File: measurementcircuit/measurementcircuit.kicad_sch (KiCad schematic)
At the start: 166 parts, among them J1 Conn_01x02, J10 Conn_01x02, J11 Conn_01x02, J12 Conn_01x02, J13 2604-3102, J14 DILB28P-223TLF, J15 Conn_01x02, J16 Conn_01x02, J17 Conn_01x02, J18 2604-3102, J19 2604-3102, J2 Conn_01x02, J20 2604-3102, J21 Conn_01x02, J22 Conn_01x02, J23 Conn_01x02, J24 Conn_01x02, J25 Conn_01x02, J26 Conn_01x02, J27 Conn_01x02, J28 Conn_01x02, J29 Conn_01x02, J3 2604-3102, J30 Conn_01x02, J31 Conn_01x02, J32 Conn_01x02, J33 Conn_01x02, J34 Conn_01x02, J35 Conn_01x02, J36 Conn_01x02, J37 Conn_01x02, J38 Conn_01x02, J39 Conn_01x02, J4 2604-3102, J40 Conn_01x02, J41 Conn_01x02, J42 Conn_01x02, J43 DILB28P-223TLF, J44 2601-1102, J45 2601-1108, J46 2601-1108, J47 Conn_01x02, J48 Conn_01x02, J49 Conn_01x02, J5 2604-3102, J50 2604-3102, J51 Conn_01x02, J52 Conn_01x02, J53 Conn_01x02, J54 Conn_01x02, J55 2604-3102, J56 Conn_01x02, J57 Conn_01x02, J58 Conn_01x02, J59 Conn_01x02, J6 2604-3102, J60 2601-1108, J61 2604-3102, J62 Conn_01x02, J63 Conn_01x02, J64 Conn_01x02, J65 Conn_01x02, J66 2604-3102, J67 Conn_01x02, J68 Conn_01x02, J69 Conn_01x02, J7 2604-3102, J70 Conn_01x02, J71 2604-3102, J72 Conn_01x02, J73 Conn_01x02, J74 Conn_01x02, J75 Conn_01x02, J76 2604-3102, J77 Conn_01x02, J78 Conn_01x02, J79 Conn_01x02, J8 Conn_01x02, J80 Conn_01x02, J81 2604-3102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

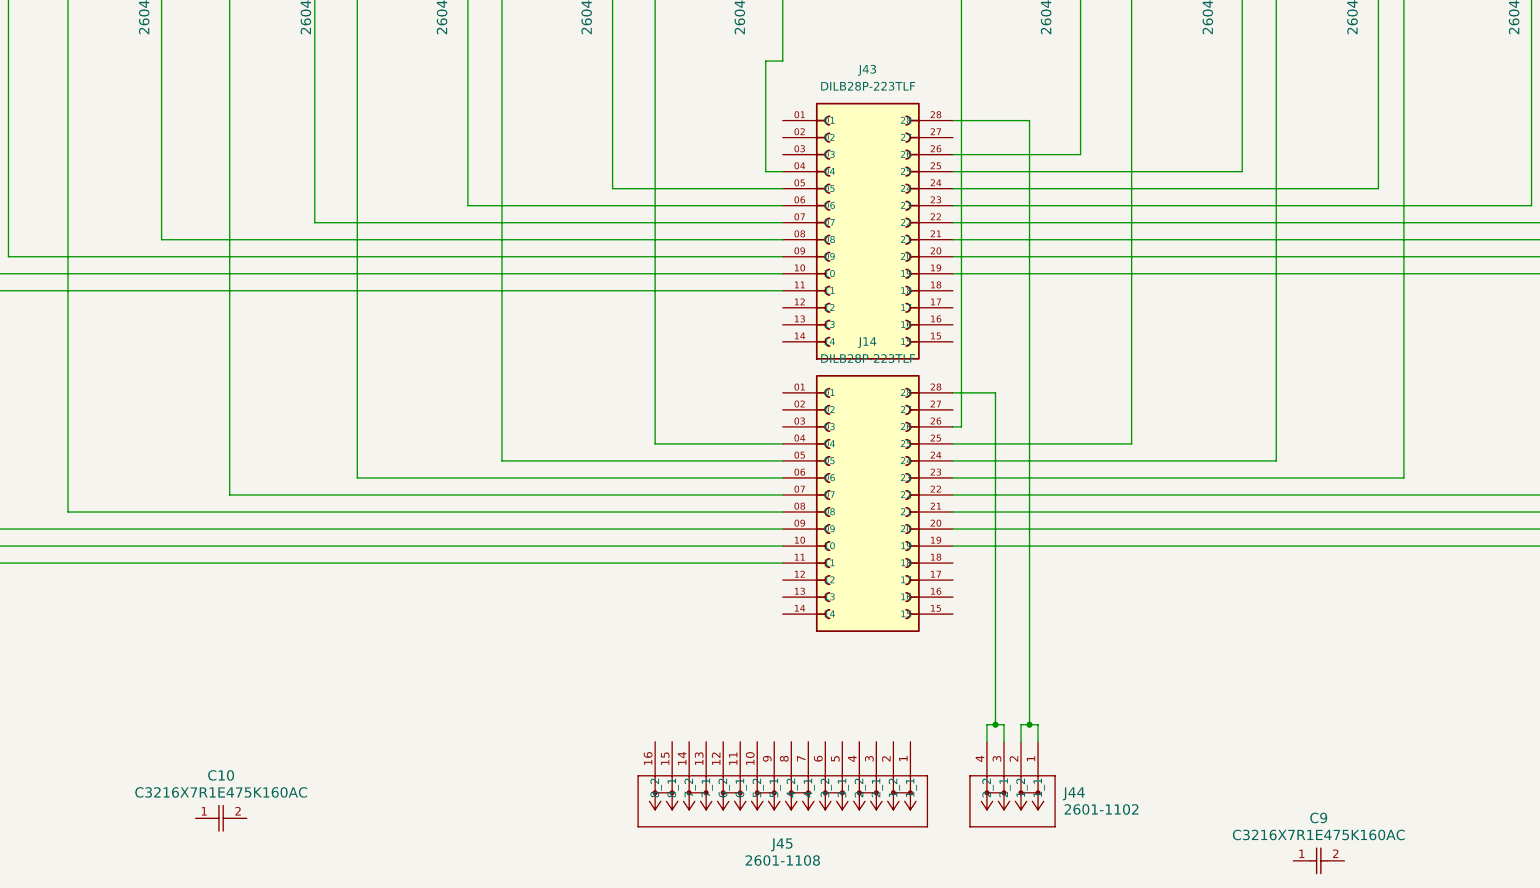
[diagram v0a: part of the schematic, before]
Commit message: Schematic Complete
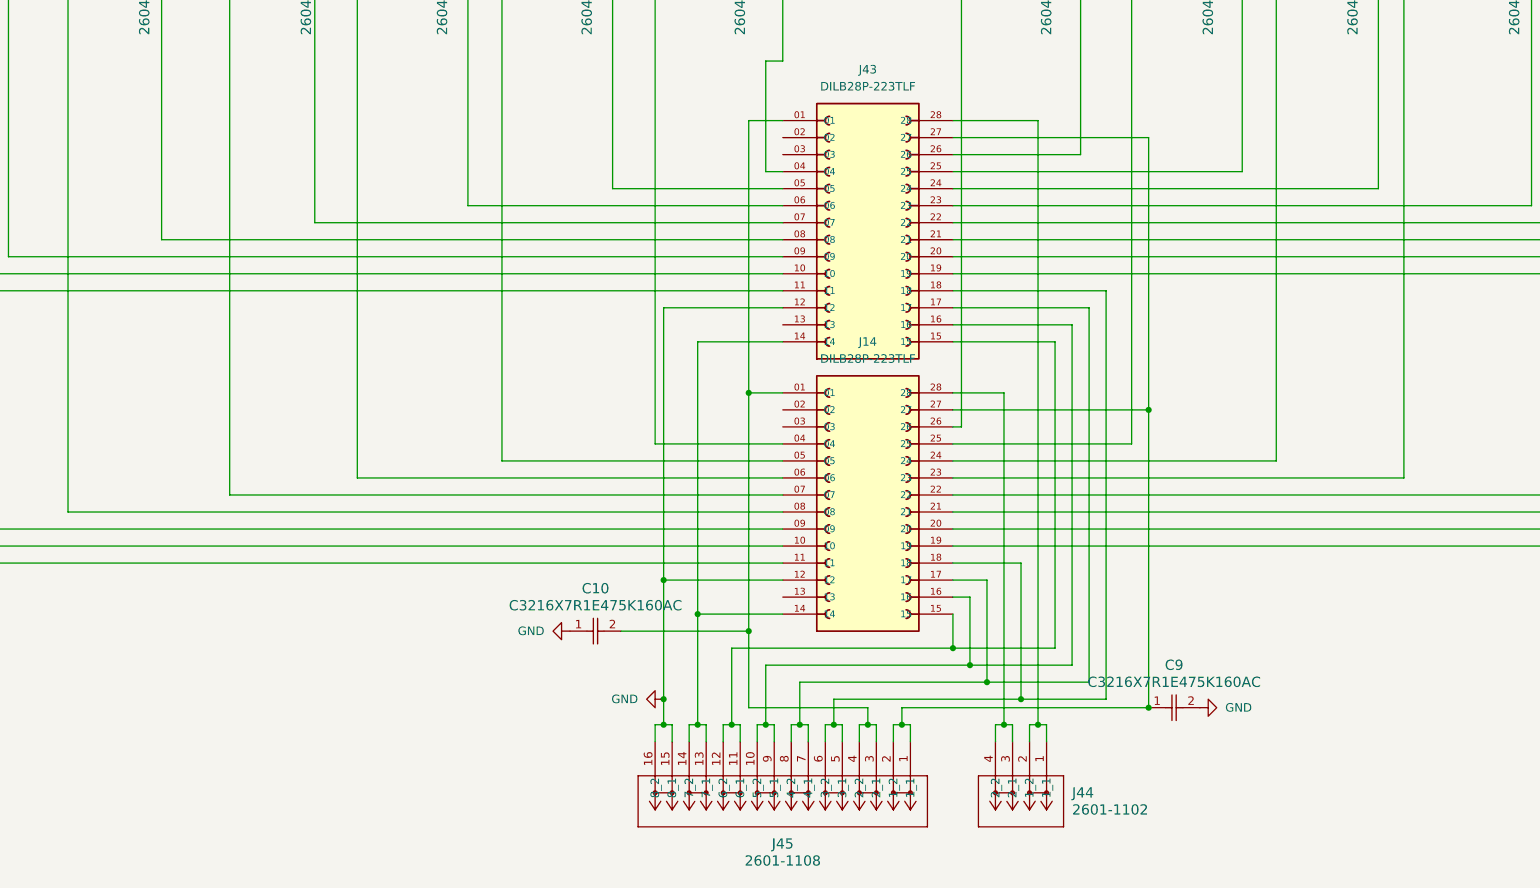
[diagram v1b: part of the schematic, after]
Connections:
- net GND: now also C10.1, C9.2, J14.12, J43.12, J45.15 (8_1), J45.16 (8_2)
- net at C10.2: now also J14.01, J43.01, J45.3 (2_1), J45.4 (2_2)
- net at J43.14: now also J14.14, J45.13 (7_1), J45.14 (7_2)
- net at J43.15: now also J14.15, J45.11 (6_1), J45.12 (6_2)
- net at J43.16: now also J14.16, J45.10 (5_2), J45.9 (5_1)
- net at J43.17: now also J14.17, J45.7 (4_1), J45.8 (4_2)
- net at J43.18: now also J14.18, J45.5 (3_1), J45.6 (3_2)
- net at J43.27: now also C9.1, J14.27, J45.1 (1_1), J45.2 (1_2)
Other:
- moved on the sheet: C10, C9, J44
